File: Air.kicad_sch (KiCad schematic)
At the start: 29 parts, among them J10 USB_C_Receptacle_USB2.0_14P, J11 Conn_ST_STDC14, J12 CAN, J13 CAN, J9 24V IN, SW1 NRST, U10 CH340E, U11 STM32F303K8Tx, U12 TJA1441, U9 NJM12877

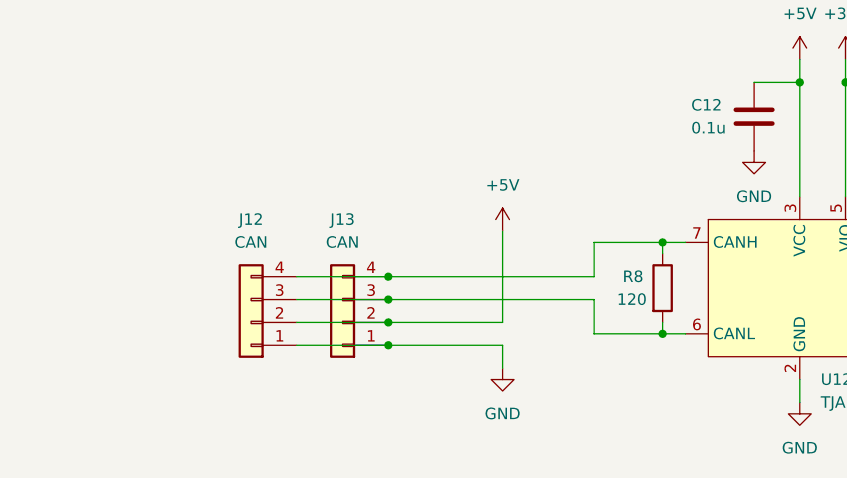
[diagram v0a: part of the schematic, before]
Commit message: chore: Update Air.kicad_pro configuration file
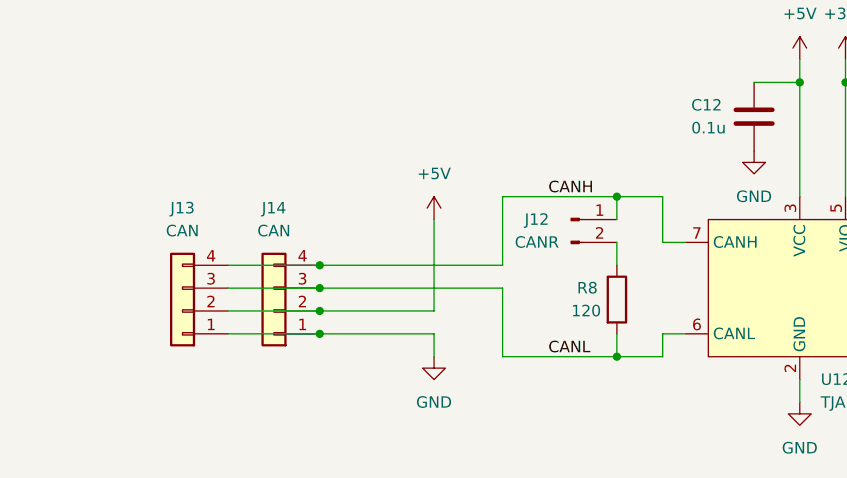
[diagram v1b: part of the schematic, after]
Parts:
- added J12: CANR, Connector_PinHeader_2.54mm:PinHeader_1x02_P2.54mm_Vertical, symbol Connector:Conn_01x02_Pin
- renumbered J12 to J13, J13 to J14
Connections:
- net CANL: now reaches J13.3 (Pin_3), J14.3 (Pin_3), R8.2, U12.6 (CANL)
- net CANH: now reaches J13.4 (Pin_4), J14.4 (Pin_4), U12.7 (CANH)
- net CANH: now also J12.1 (Pin_1); no longer R8.1
- new net: J12.2 (Pin_2), R8.1
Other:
- moved on the sheet: J13, J14, R8
